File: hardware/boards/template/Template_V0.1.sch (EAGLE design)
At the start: 2 parts

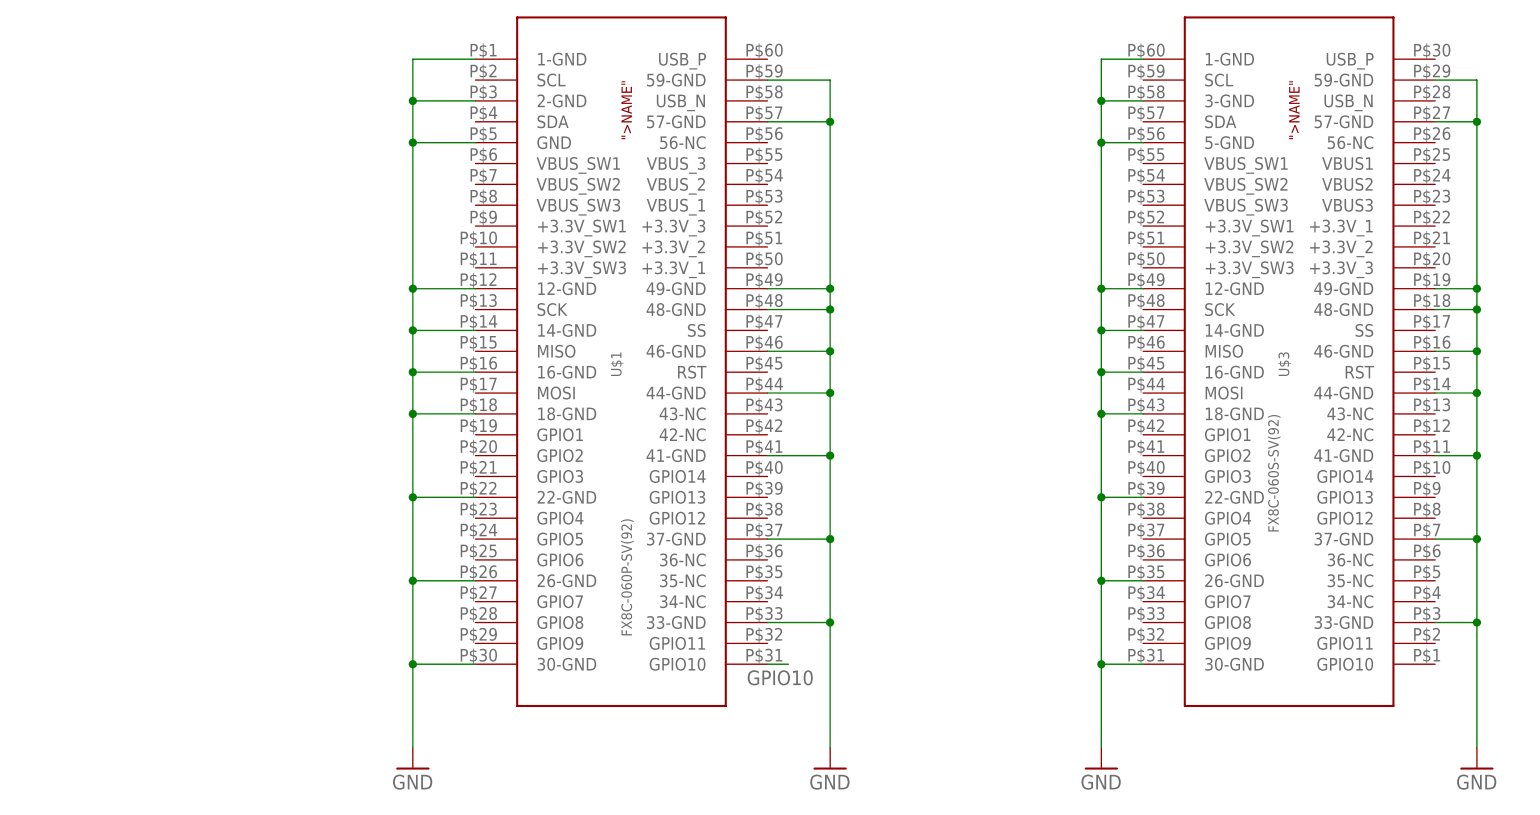
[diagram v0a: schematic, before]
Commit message: Updating template, wip
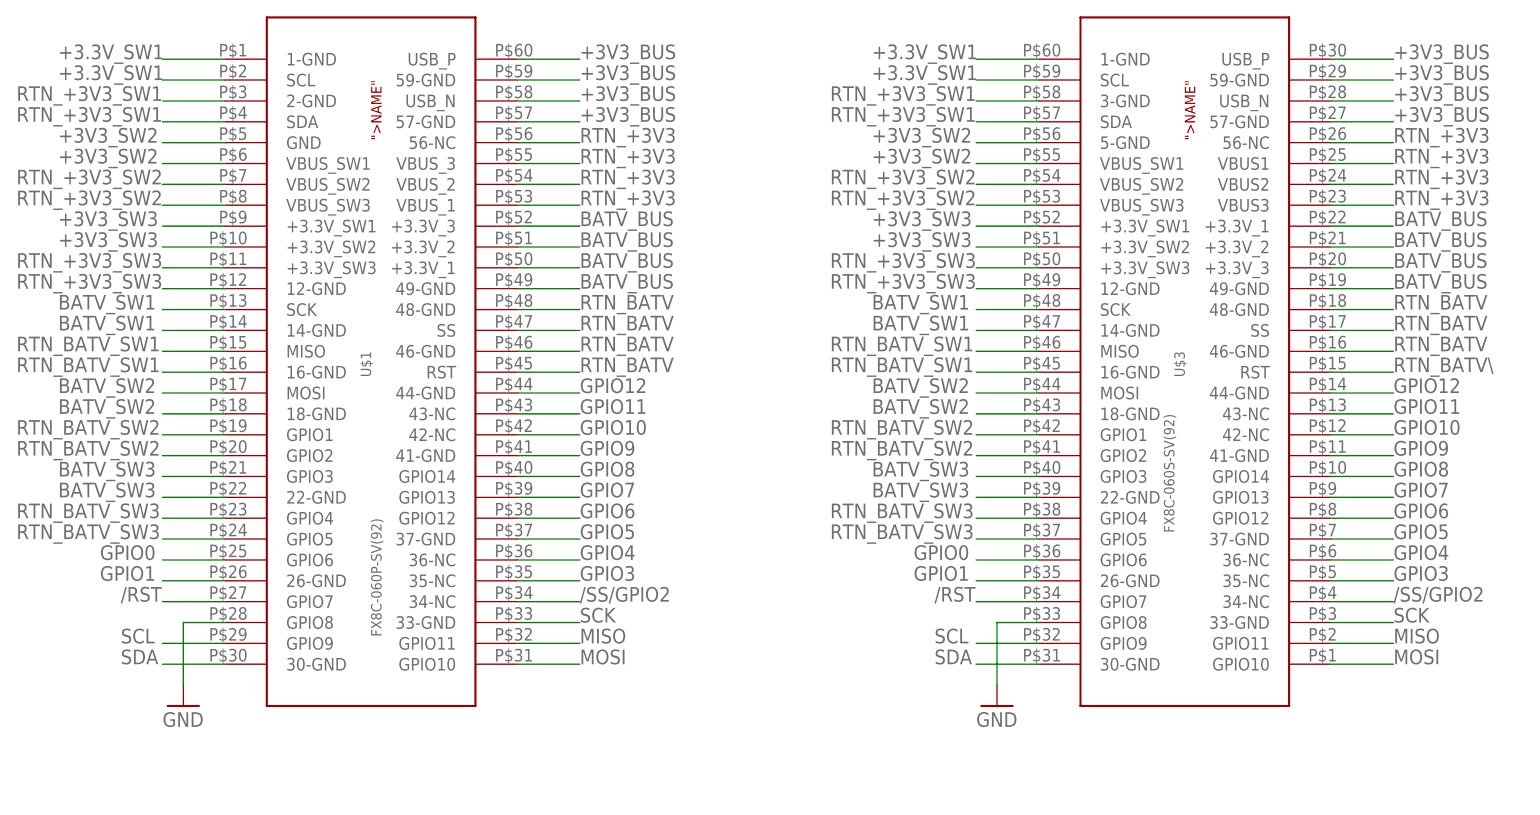
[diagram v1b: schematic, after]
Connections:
- new net +3.3V_SW1: U$1.1-GND, U$1.SCL, U$3.1-GND, U$3.SCL
- new net +3V3_BUS: U$1.57-GND, U$1.59-GND, U$1.USB_N, U$1.USB_P
- new net +3V3_SW2: U$1.GND, U$1.VBUS_SW1, U$3.5-GND, U$3.VBUS_SW1
- new net +3V3_SW3: U$1.+3.3V_SW1, U$1.+3.3V_SW2, U$3.+3.3V_SW1, U$3.+3.3V_SW2
- new net /RST: U$1.GPIO7, U$3.GPIO7
- new net /SS/GPIO2: U$1.34-NC
- new net BATV_BUS: U$1.+3.3V_1, U$1.+3.3V_2, U$1.+3.3V_3, U$1.49-GND
- new net BATV_SW1: U$1.14-GND, U$1.SCK, U$3.14-GND, U$3.SCK
- new net BATV_SW2: U$1.18-GND, U$1.MOSI, U$3.18-GND, U$3.MOSI
- new net BATV_SW3: U$1.22-GND, U$1.GPIO3, U$3.22-GND, U$3.GPIO3
- new net GPIO0: U$1.GPIO6, U$3.GPIO6
- new net GPIO1: U$1.26-GND, U$3.26-GND
- new net GPIO11: U$1.43-NC
- new net GPIO12: U$1.44-GND
- new net GPIO3: U$1.35-NC
- new net GPIO4: U$1.36-NC
- new net GPIO5: U$1.37-GND
- new net GPIO6: U$1.GPIO12
- new net GPIO7: U$1.GPIO13
- new net GPIO8: U$1.GPIO14
- new net GPIO9: U$1.41-GND
- new net MISO: U$1.GPIO11
- new net MOSI: U$1.GPIO10
- new net RTN_+3V3: U$1.56-NC, U$1.VBUS_1, U$1.VBUS_2, U$1.VBUS_3
- new net RTN_+3V3_SW1: U$1.2-GND, U$1.SDA, U$3.3-GND, U$3.SDA
- new net RTN_+3V3_SW2: U$1.VBUS_SW2, U$1.VBUS_SW3, U$3.VBUS_SW2, U$3.VBUS_SW3
- new net RTN_+3V3_SW3: U$1.+3.3V_SW3, U$1.12-GND, U$3.+3.3V_SW3, U$3.12-GND
- new net RTN_BATV: U$1.46-GND, U$1.48-GND, U$1.RST, U$1.SS
- new net RTN_BATV_SW1: U$1.16-GND, U$1.MISO, U$3.16-GND, U$3.MISO
- new net RTN_BATV_SW2: U$1.GPIO1, U$1.GPIO2, U$3.GPIO1, U$3.GPIO2
- new net RTN_BATV_SW3: U$1.GPIO4, U$1.GPIO5, U$3.GPIO4, U$3.GPIO5
- new net SCK: U$1.33-GND
- new net SCL: U$1.GPIO9, U$3.GPIO9
- new net SDA: U$1.30-GND, U$3.30-GND
- net GND: now also U$1.GPIO8, U$3.GPIO8; no longer U$1.1-GND, U$1.12-GND, U$1.14-GND, U$1.16-GND, U$1.18-GND, U$1.2-GND, U$1.22-GND, U$1.26-GND, U$1.30-GND, U$1.33-GND, U$1.37-GND, U$1.41-GND, U$1.44-GND, U$1.46-GND, U$1.48-GND, U$1.49-GND, U$1.57-GND, U$1.59-GND, U$1.GND, U$3.1-GND, U$3.12-GND, U$3.14-GND, U$3.16-GND, U$3.18-GND, U$3.22-GND, U$3.26-GND, U$3.3-GND, U$3.30-GND, U$3.33-GND, U$3.37-GND, U$3.41-GND, U$3.44-GND, U$3.46-GND, U$3.48-GND, U$3.49-GND, U$3.5-GND, U$3.57-GND, U$3.59-GND
- net GPIO10: now also U$1.42-NC; no longer U$1.GPIO10
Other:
- moved on the sheet: U$1, U$3
